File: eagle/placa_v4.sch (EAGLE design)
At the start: 20 parts, among them IC1 7805

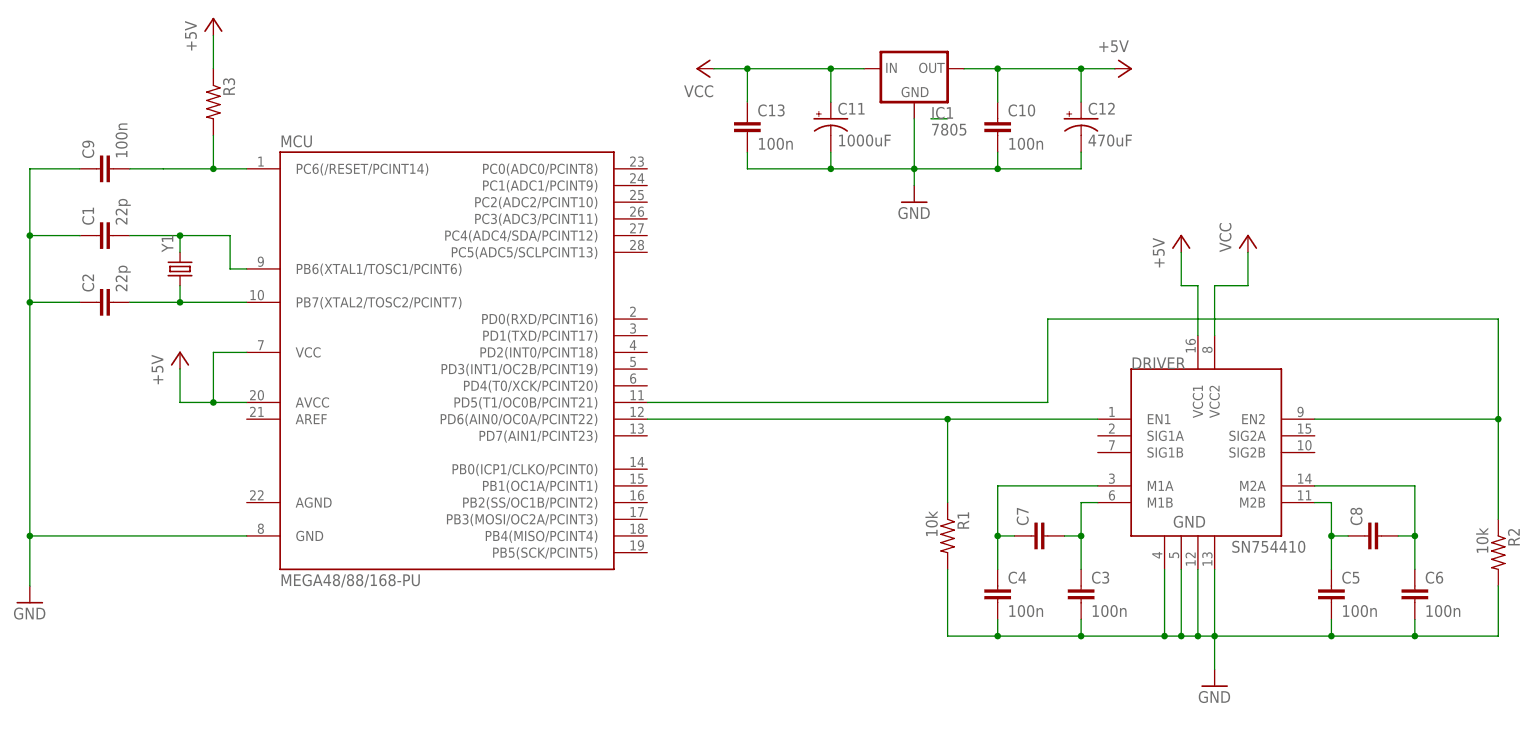
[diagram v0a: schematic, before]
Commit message: Circuito
git-svn-id: https://mbs-bot.googlecode.com/svn/trunk@202 3c29fe3e-da84-11de-ae71-c59d11f48c9c
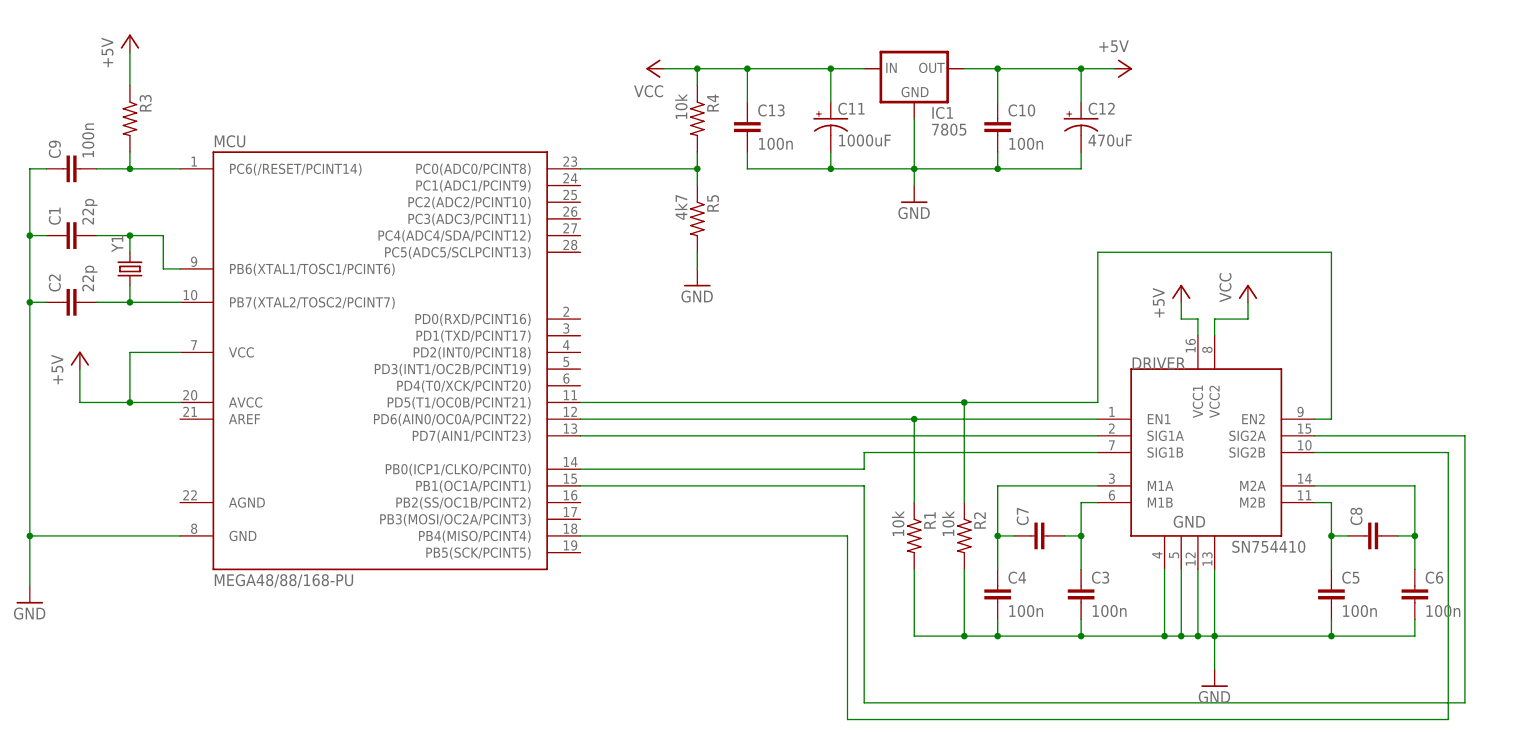
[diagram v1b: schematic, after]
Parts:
- added R4: 10k, SparkFun:RESISTORPTH-1/2W
- added R5: 4k7, SparkFun:RESISTORPTH-1/2W
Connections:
- new net N$11: DRIVER.SIG1A, MCU.PD7(AIN1/PCINT23)
- new net N$12: DRIVER.SIG1B, MCU.PB0(ICP1/CLKO/PCINT0)
- new net N$13: DRIVER.SIG2B, MCU.PB4(MISO/PCINT4)
- new net N$14: DRIVER.SIG2A, MCU.PB1(OC1A/PCINT1)
- new net N$9: MCU.PC0(ADC0/PCINT8), R4.2, R5.1
- net GND: now also R5.2
- net VCC: now also R4.1
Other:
- moved on the sheet: C1, C2, C9, MCU, R1, R2, R3, Y1
